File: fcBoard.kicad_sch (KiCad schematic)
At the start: 0 parts

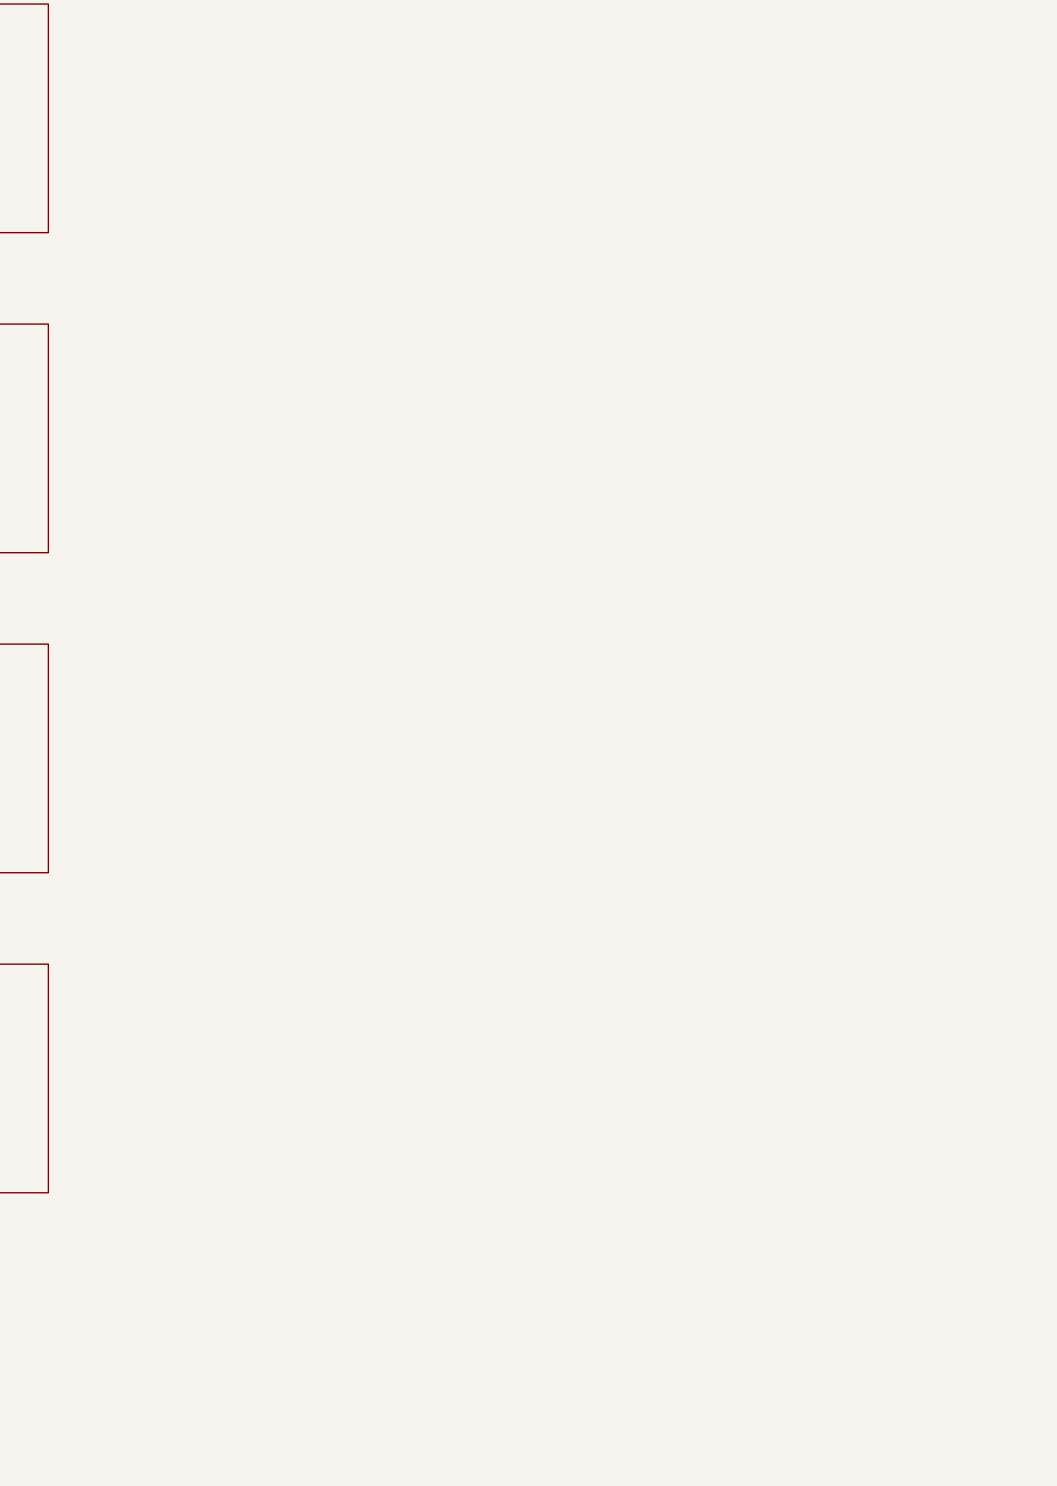
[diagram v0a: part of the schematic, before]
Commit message: 45
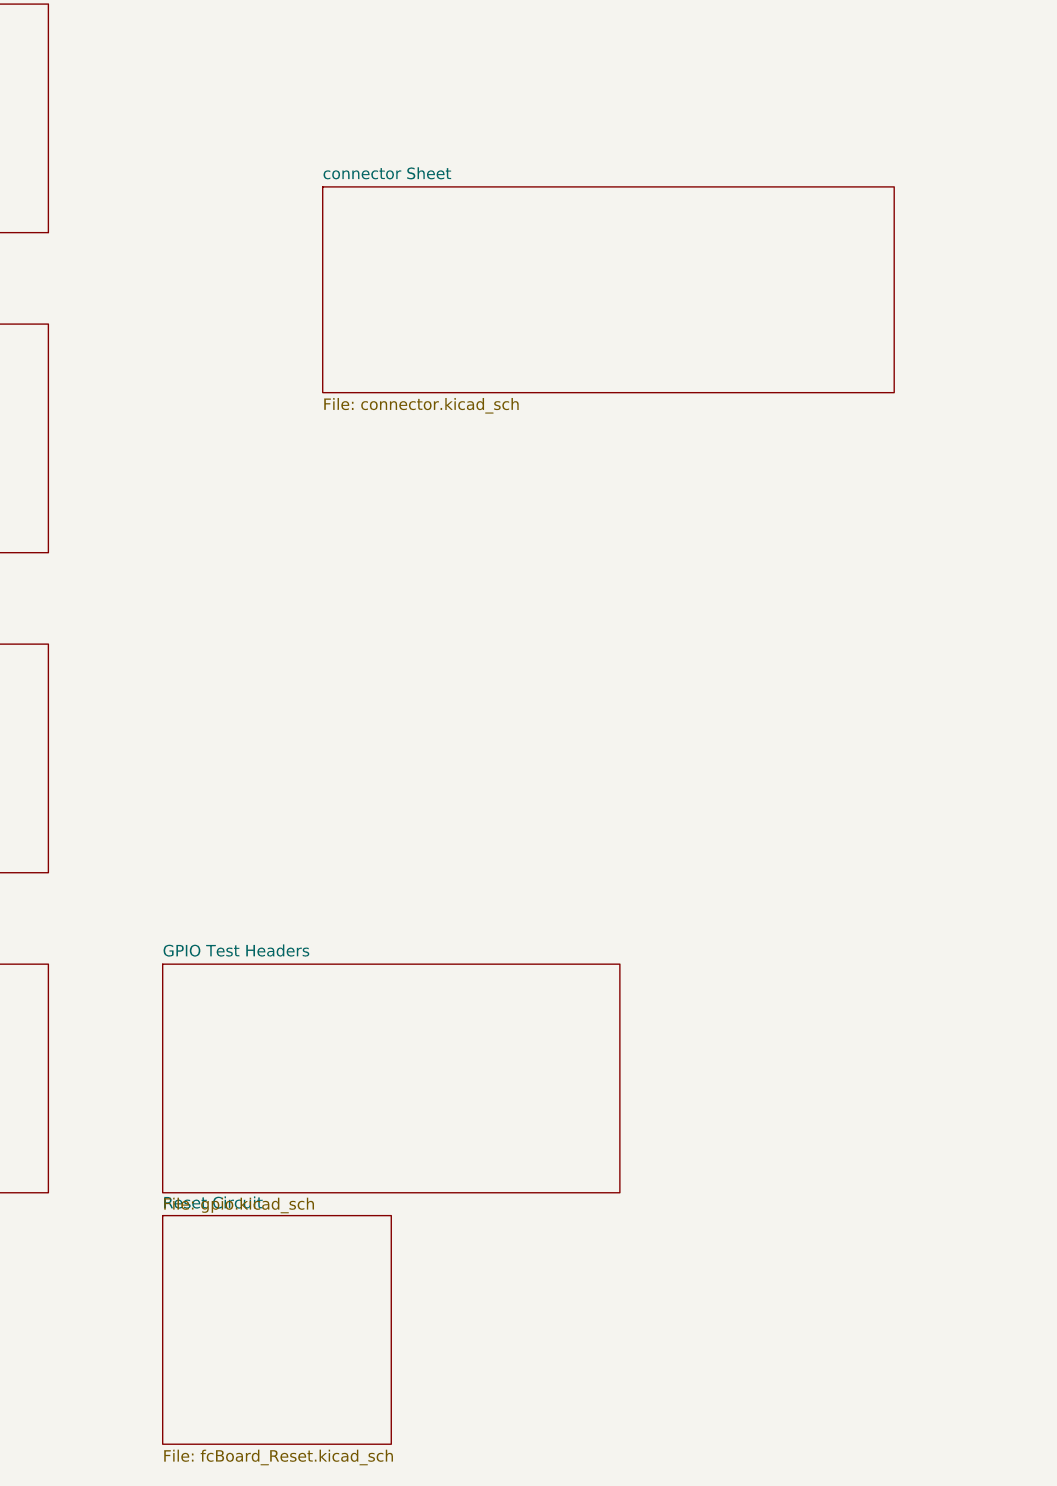
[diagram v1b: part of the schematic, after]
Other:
- added sheet GPIO Test Headers (gpio.kicad_sch)
- added sheet Reset Circuit (fcBoard_Reset.kicad_sch)
- added sheet connector Sheet (connector.kicad_sch)
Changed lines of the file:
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@@
+	)
+	(sheet
+		(at 106.68 139.7)
+		(size 63.5 22.86)
+		(exclude_from_sim no)
+		(in_bom yes)
+		(on_board yes)
+		(dnp no)
+		(fields_autoplaced yes)
+		(stroke
+			(width 0.1524)
+			(type solid)
+		)
+		(fill
+			(color 0 0 0 0.0000)
+		)
+		(property "Sheetname" "connector Sheet"
+			(at 106.68 138.9884 0)
+			(effects
+				(font
+					(size 1.27 1.27)
+				)
+				(justify left bottom)
+			)
+		)
+		(property "Sheetfile" "connector.kicad_sch"
+			(at 106.68 163.1446 0)
+			(effects
+				(font
+					(size 1.27 1.27)
+				)
+				(justify left top)
+			)
+		)
+		(instances
+			(project "fcBoard"
+				(path "/e63e39d7-6ac0-4ffd-8aa3-1841a4541b55"
+					(page "7")
+				)
+			)
+		)
+	)
+	(sheet
+		(at 88.9 254)
+		(size 25.4 25.4)
+		(exclude_from_sim no)
+		(in_bom yes)
+		(on_board yes)
+		(dnp no)
+		(fields_autoplaced yes)
+		(stroke
+			(width 0.1524)
+			(type solid)
+		)
+		(fill
+			(color 255 224 194 1.0000)
+		)
+		(property "Sheetname" "Reset Circuit"
+			(at 88.9 253.3484 0)
+			(effects
+				(font
+					(size 1.27 1.27)
+				)
+				(justify left bottom)
+			)
+		)
+		(property "Sheetfile" "fcBoard_Reset.kicad_sch"
+			(at 88.9 280.0016 0)
+			(effects
+				(font
+					(size 1.27 1.27)
+				)
+				(justify left top)
+			)
+		)
+		(instances
+			(project "fcBoard"
+				(path "/e63e39d7-6ac0-4ffd-8aa3-1841a4541b55"
+					(page "9")
+				)
+			)
+		)
 	)
 	(sheet
@@
 				)
 			)
+		)
+	)
+	(sheet
+		(at 88.9 226.06)
+		(size 50.8 25.4)
+		(exclude_from_sim no)
+		(in_bom yes)
+		(on_board yes)
+		(dnp no)
+		(fields_autoplaced yes)
+		(stroke
+			(width 0.1524)
+			(type solid)
+		)
+		(fill
+			(color 194 255 224 1.0000)
+		)
+		(property "Sheetname" "GPIO Test Headers"
+			(at 88.9 225.3484 0)
+			(effects
+				(font
+					(size 1.27 1.27)
+				)
+				(justify left bottom)
+			)
+		)
+		(property "Sheetfile" "gpio.kicad_sch"
+			(at 88.9 252.0016 0)
+			(effects
+				(font
+					(size 1.27 1.27)
+				)
+				(justify left top)
+			)
+		)
+		(instances
+			(project "fcBoard"
+				(path "/e63e39d7-6ac0-4ffd-8aa3-1841a4541b55"
+					(page "8")
+				)
+			)
